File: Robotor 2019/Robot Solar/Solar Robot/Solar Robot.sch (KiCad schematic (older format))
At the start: 39 parts, among them J1 Conn_01x02, J2 Conn_01x06_Male, M1 Motor_DC, M2 Motor_DC, SW1 SW_DIP_x01, SW2 SW_Push, SW3 SW_Push, U1 ATmega328-PU, U2 ITR8307, U3 ITR8307, U4 ITR8307, U5 ITR8307, Y1 16Mhz

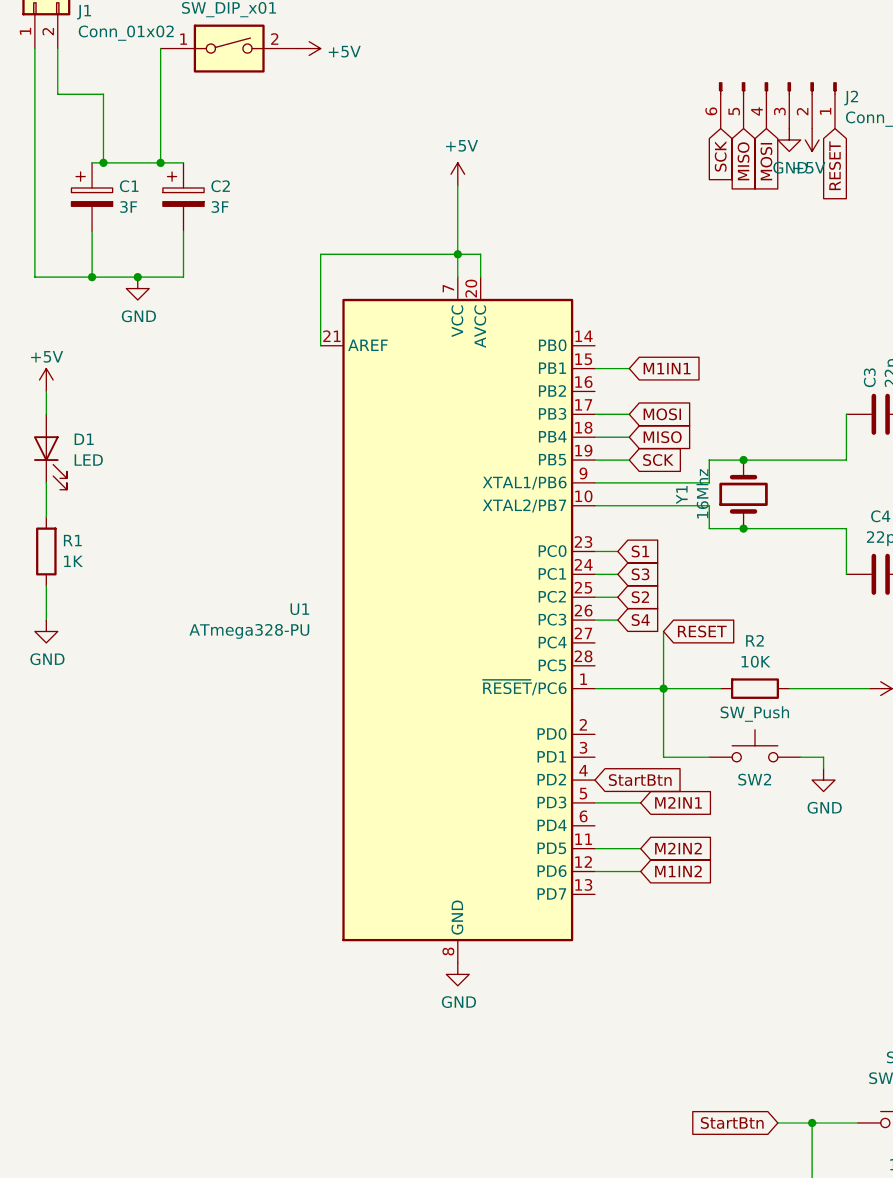
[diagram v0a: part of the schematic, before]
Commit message: no message
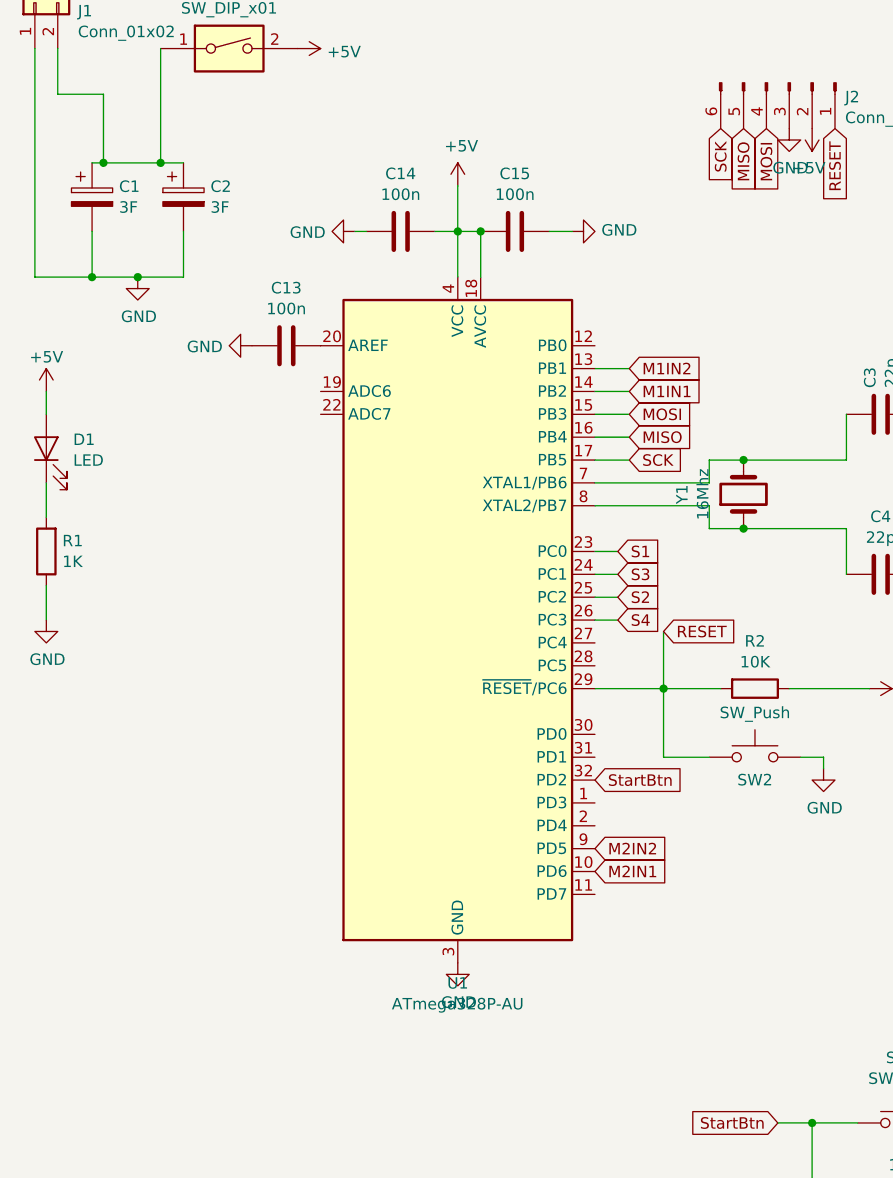
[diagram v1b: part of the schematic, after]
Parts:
- removed U1: ATmega328-PU, Package_QFP:TQFP-32_7x7mm_P0.8mm, symbol MCU_Microchip_ATmega:ATmega328-PU
- added C13, C14, C15: 100n, Capacitor_SMD:C_0805_2012Metric_Pad1.15x1.40mm_HandSolder, symbol Device:C
- added U1: ATmega328P-AU, Package_QFP:TQFP-32_7x7mm_P0.8mm, symbol MCU_Microchip_ATmega:ATmega328P-AU
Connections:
- net +5V: now also C14.1, C15.2, U1.18 (AVCC), U1.4 (VCC), U1.6 (VCC)
- net GND: now also C13.2, C14.2, C15.1, U1.21 (GND), U1.3 (GND), U1.5 (GND)
- net M1IN1: now also U1.14 (PB2)
- net M1IN2: now also U1.13 (PB1)
- net M2IN1: now also U1.10 (PD6)
- net M2IN2: now also U1.9 (PD5)
- net MISO: now also U1.16 (PB4)
- net MOSI: now also U1.15 (PB3)
- net RESET: now also U1.29 (~RESET~/PC6)
- net S1: now also U1.23 (PC0)
- net S2: now also U1.25 (PC2)
- net S3: now also U1.24 (PC1)
- net S4: now also U1.26 (PC3)
- net SCK: now also U1.17 (PB5)
- net StartBtn: now also U1.32 (PD2)
- net at C4.2, Y1.1: now also U1.8 (XTAL2/PB7)
- net at C3.1, Y1.2: now also U1.7 (XTAL1/PB6)
- new net: C13.1, U1.20 (AREF)
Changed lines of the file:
@@
 Wire Wire Line
 	4650 2850 4650 3200
-Wire Wire Line
-	2050 2200 2050 1800
-Wire Wire Line
-	2050 1800 2650 1800
-Wire Wire Line
-	2750 1800 2750 1900
-Wire Wire Line
-	2650 1900 2650 1800
-Connection ~ 2650 1800
-Wire Wire Line
-	2650 1800 2750 1800
-Wire Wire Line
-	2650 1500 2650 1800
 $Comp
 L power:+5V #PWR0103
@@
 	0    1    1    0
 $EndComp
-Wire Wire Line
-	3250 3700 3550 3700
 $Comp
 L power:+5V #PWR0105
@@
 	1    0    0    -1
 $EndComp
-Text GLabel 3250 4100 2    50   Input ~ 0
-StartBtn
 Text GLabel 4050 5600 0    50   Input ~ 0
 StartBtn
@@
 Text GLabel 10050 800  1    50   Input ~ 0
 S4
+Text GLabel 3400 2400 2    50   Input ~ 0
+M1IN1
 Text GLabel 3400 2300 2    50   Input ~ 0
-M1IN1
-Text GLabel 3450 4500 2    50   Input ~ 0
 M1IN2
-Wire Wire Line
-	3250 4500 3450 4500
 Wire Wire Line
 	3250 2300 3400 2300
@@
 Wire Wire Line
 	8500 5000 8600 5000
-Text GLabel 3450 4200 2    50   Input ~ 0
+Text GLabel 3250 4500 2    50   Input ~ 0
 M2IN1
-Text GLabel 3450 4400 2    50   Input ~ 0
+Text GLabel 3250 4400 2    50   Input ~ 0
 M2IN2
-Wire Wire Line
-	3250 4200 3450 4200
-Wire Wire Line
-	3250 4400 3450 4400
-$Comp
-L MCU_Microchip_ATmega:ATmega328-PU U1
-U 1 1 5D348BDA
+$Comp
+L MCU_Microchip_ATmega:ATmega328P-AU U1
+U 1 1 5D56EBEE
 P 2650 3400
-F 0 "U1" H 2006 3446 50  0000 R CNN
-F 1 "ATmega328-PU" H 2006 3355 50  0000 R CNN
+F 0 "U1" H 2650 1811 50  0000 C CNN
+F 1 "ATmega328P-AU" H 2650 1720 50  0000 C CNN
 F 2 "Package_QFP:TQFP-32_7x7mm_P0.8mm" H 2650 3400 50  0001 C CIN
 F 3 "http://ww1.microchip.com/downloads/en/DeviceDoc/ATmega328_P%20AVR%20MCU%20with%20picoPower%20Technology%20Data%20Sheet%2040001984A.pdf" H 2650 3400 50  0001 C CNN
@@
 	1    0    0    -1
 $EndComp
+Wire Wire Line
+	2650 1500 2650 1700
+$Comp
+L Device:C C15
+U 1 1 5D57E1CC
+P 2900 1700
+F 0 "C15" V 2648 1700 50  0000 C CNN
+F 1 "100n" V 2739 1700 50  0000 C CNN
+F 2 "Capacitor_SMD:C_0805_2012Metric_Pad1.15x1.40mm_HandSolder" H 2938 1550 50  0001 C CNN
+F 3 "~" H 2900 1700 50  0001 C CNN
+	1    2900 1700
+	0    1    1    0
+$EndComp
+Wire Wire Line
+	2750 1900 2750 1700
+Wire Wire Line
+	2750 1700 2650 1700
+Connection ~ 2750 1700
+Connection ~ 2650 1700
+Wire Wire Line
+	2650 1700 2650 1900
+Wire Wire Line
+	3050 1700 3150 1700
+$Comp
+L power:GND #PWR0127
+U 1 1 5D591C28
+P 3150 1700
+F 0 "#PWR0127" H 3150 1450 50  0001 C CNN
+F 1 "GND" V 3155 1572 50  0000 R CNN
+F 2 "" H 3150 1700 50  0001 C CNN
+F 3 "" H 3150 1700 50  0001 C CNN
+	1    3150 1700
+	0    -1   -1   0
+$EndComp
+$Comp
+L Device:C C13
+U 1 1 5D597E66
+P 1900 2200
+F 0 "C13" V 1648 2200 50  0000 C CNN
+F 1 "100n" V 1739 2200 50  0000 C CNN
+F 2 "Capacitor_SMD:C_0805_2012Metric_Pad1.15x1.40mm_HandSolder" H 1938 2050 50  0001 C CNN
+F 3 "~" H 1900 2200 50  0001 C CNN
+	1    1900 2200
+	0    1    1    0
+$EndComp
+$Comp
+L power:GND #PWR0128
+U 1 1 5D598B6F
+P 1750 2200
+F 0 "#PWR0128" H 1750 1950 50  0001 C CNN
+F 1 "GND" V 1755 2072 50  0000 R CNN
+F 2 "" H 1750 2200 50  0001 C CNN
+F 3 "" H 1750 2200 50  0001 C CNN
+	1    1750 2200
+	0    1    1    0
+$EndComp
+$Comp
+L Device:C C14
+U 1 1 5D598D04
+P 2400 1700
+F 0 "C14" V 2148 1700 50  0000 C CNN
+F 1 "100n" V 2239 1700 50  0000 C CNN
+F 2 "Capacitor_SMD:C_0805_2012Metric_Pad1.15x1.40mm_HandSolder" H 2438 1550 50  0001 C CNN
+F 3 "~" H 2400 1700 50  0001 C CNN
+	1    2400 1700
+	0    1    1    0
+$EndComp
+Wire Wire Line
+	2650 1700 2550 1700
+$Comp
+L power:GND #PWR0129
+U 1 1 5D59F251
+P 2200 1700
+F 0 "#PWR0129" H 2200 1450 50  0001 C CNN
+F 1 "GND" V 2205 1572 50  0000 R CNN
+F 2 "" H 2200 1700 50  0001 C CNN
+F 3 "" H 2200 1700 50  0001 C CNN
+	1    2200 1700
+	0    1    1    0
+$EndComp
+Wire Wire Line
+	2200 1700 2250 1700
+Wire Wire Line
+	3250 2400 3400 2400
+Wire Wire Line
+	3250 3700 3550 3700
+Text GLabel 3250 4100 2    50   Input ~ 0
+StartBtn
 $EndSCHEMATC

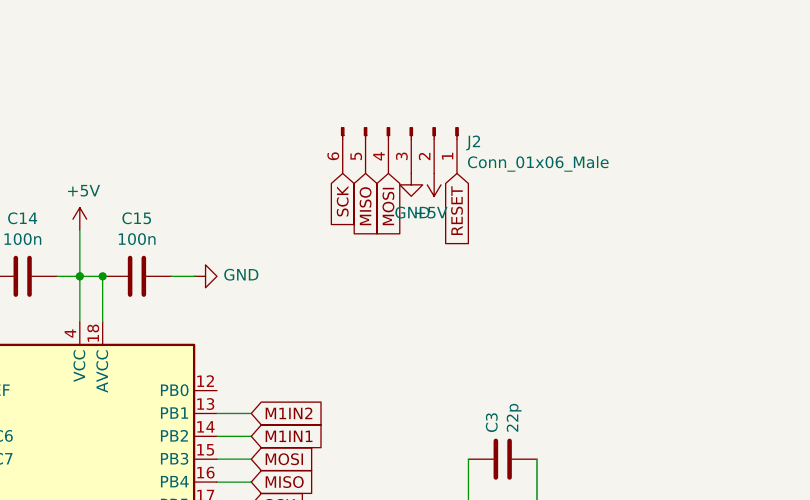
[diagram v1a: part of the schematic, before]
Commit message: Honestly I don't even remember
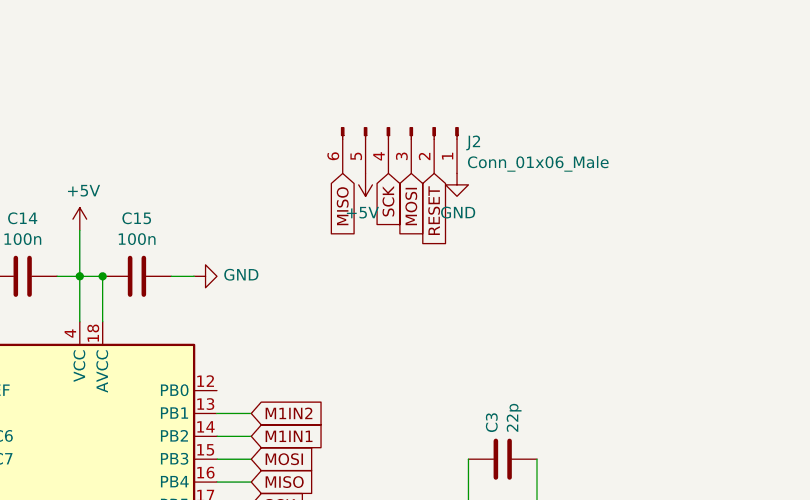
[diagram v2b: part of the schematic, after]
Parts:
- J2: footprint Connector_PinHeader_2.54mm:PinHeader_1x06_P2.54mm_Vertical -> Connector_PinSocket_2.54mm:PinSocket_2x03_P2.54mm_Vertical
- SW2, SW3: footprint Button_Switch_SMD:SW_Push_1P1T_NO_6x6mm_H9.5mm -> Button_Switch_SMD:SW_SPST_CK_RS282G05A3
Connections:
- net +5V: now also J2.5 (Pin_5); no longer J2.2 (Pin_2)
- net GND: now also J2.1 (Pin_1); no longer J2.3 (Pin_3)
- net MISO: now also J2.6 (Pin_6); no longer J2.5 (Pin_5)
- net MOSI: now also J2.3 (Pin_3); no longer J2.4 (Pin_4)
- net RESET: now also J2.2 (Pin_2); no longer J2.1 (Pin_1)
- net SCK: now also J2.4 (Pin_4); no longer J2.6 (Pin_6)
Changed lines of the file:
@@
 F 0 "SW2" H 3950 3900 50  0000 C CNN
 F 1 "SW_Push" H 3950 4194 50  0000 C CNN
-F 2 "Button_Switch_SMD:SW_Push_1P1T_NO_6x6mm_H9.5mm" H 3950 4200 50  0001 C CNN
+F 2 "Button_Switch_SMD:SW_SPST_CK_RS282G05A3" H 3950 4200 50  0001 C CNN
 F 3 "~" H 3950 4200 50  0001 C CNN
 	1    3950 4000
@@
 F 0 "J2" V 4162 1294 50  0000 L CNN
 F 1 "Conn_01x06_Male" V 4253 1294 50  0000 L CNN
-F 2 "Connector_PinHeader_2.54mm:PinHeader_1x06_P2.54mm_Vertical" H 4100 1050 50  0001 C CNN
+F 2 "Connector_PinSocket_2.54mm:PinSocket_2x03_P2.54mm_Vertical" H 4100 1050 50  0001 C CNN
 F 3 "~" H 4100 1050 50  0001 C CNN
 	1    4100 1050
@@
 Wire Wire Line
 	3250 2700 3400 2700
-Text GLabel 4000 1250 3    50   Input ~ 0
+Text GLabel 4100 1250 3    50   Input ~ 0
 MOSI
-Text GLabel 3900 1250 3    50   Input ~ 0
+Text GLabel 3800 1250 3    50   Input ~ 0
 MISO
-Text GLabel 3800 1250 3    50   Input ~ 0
-SCK
 $Comp
 L power:GND #PWR0107
 U 1 1 5D372DC5
-P 4100 1250
-F 0 "#PWR0107" H 4100 1000 50  0001 C CNN
-F 1 "GND" H 4105 1077 50  0000 C CNN
-F 2 "" H 4100 1250 50  0001 C CNN
-F 3 "" H 4100 1250 50  0001 C CNN
-	1    4100 1250
-	1    0    0    -1
-$EndComp
-$Comp
-L power:+5V #PWR0108
-U 1 1 5D373435
-P 4200 1250
-F 0 "#PWR0108" H 4200 1100 50  0001 C CNN
-F 1 "+5V" H 4215 1423 50  0000 C CNN
-F 2 "" H 4200 1250 50  0001 C CNN
-F 3 "" H 4200 1250 50  0001 C CNN
-	1    4200 1250
-	-1   0    0    1
+P 4300 1250
+F 0 "#PWR0107" H 4300 1000 50  0001 C CNN
+F 1 "GND" H 4305 1077 50  0000 C CNN
+F 2 "" H 4300 1250 50  0001 C CNN
+F 3 "" H 4300 1250 50  0001 C CNN
+	1    4300 1250
+	1    0    0    -1
 $EndComp
 Text GLabel 3550 3450 2    50   Input ~ 0
 RESET
-Text GLabel 4300 1250 3    50   Input ~ 0
+Text GLabel 4200 1250 3    50   Input ~ 0
 RESET
 $Comp
@@
 F 0 "SW3" H 4600 5885 50  0000 C CNN
 F 1 "SW_Push" H 4600 5794 50  0000 C CNN
-F 2 "Button_Switch_SMD:SW_Push_1P1T_NO_6x6mm_H9.5mm" H 4600 5800 50  0001 C CNN
+F 2 "Button_Switch_SMD:SW_SPST_CK_RS282G05A3" H 4600 5800 50  0001 C CNN
 F 3 "~" H 4600 5800 50  0001 C CNN
 	1    4600 5600
@@
 Text GLabel 3250 4100 2    50   Input ~ 0
 StartBtn
+Text GLabel 4000 1250 3    50   Input ~ 0
+SCK
+$Comp
+L power:+5V #PWR0108
+U 1 1 5D373435
+P 3900 1250
+F 0 "#PWR0108" H 3900 1100 50  0001 C CNN
+F 1 "+5V" H 3915 1423 50  0000 C CNN
+F 2 "" H 3900 1250 50  0001 C CNN
+F 3 "" H 3900 1250 50  0001 C CNN
+	1    3900 1250
+	-1   0    0    1
+$EndComp
 $EndSCHEMATC
